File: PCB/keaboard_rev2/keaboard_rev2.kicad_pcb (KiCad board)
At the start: 2 copper layers, 141.9 x 93.7 mm, 61 parts, among them K01 KEYSW, K02 KEYSW, K03 KEYSW, K04 KEYSW, K05 KEYSW, K06 KEYSW, K07 KEYSW, K08 KEYSW, K09 KEYSW, K10 KEYSW, K11 KEYSW, K12 KEYSW, K13 KEYSW, K14 KEYSW, K15 KEYSW, K16 KEYSW, K17 KEYSW, K18 KEYSW, K19 KEYSW, K20 KEYSW, K21 KEYSW, K22 KEYSW, K23 KEYSW, K24 KEYSW, K25 KEYSW, U1 ProMicro

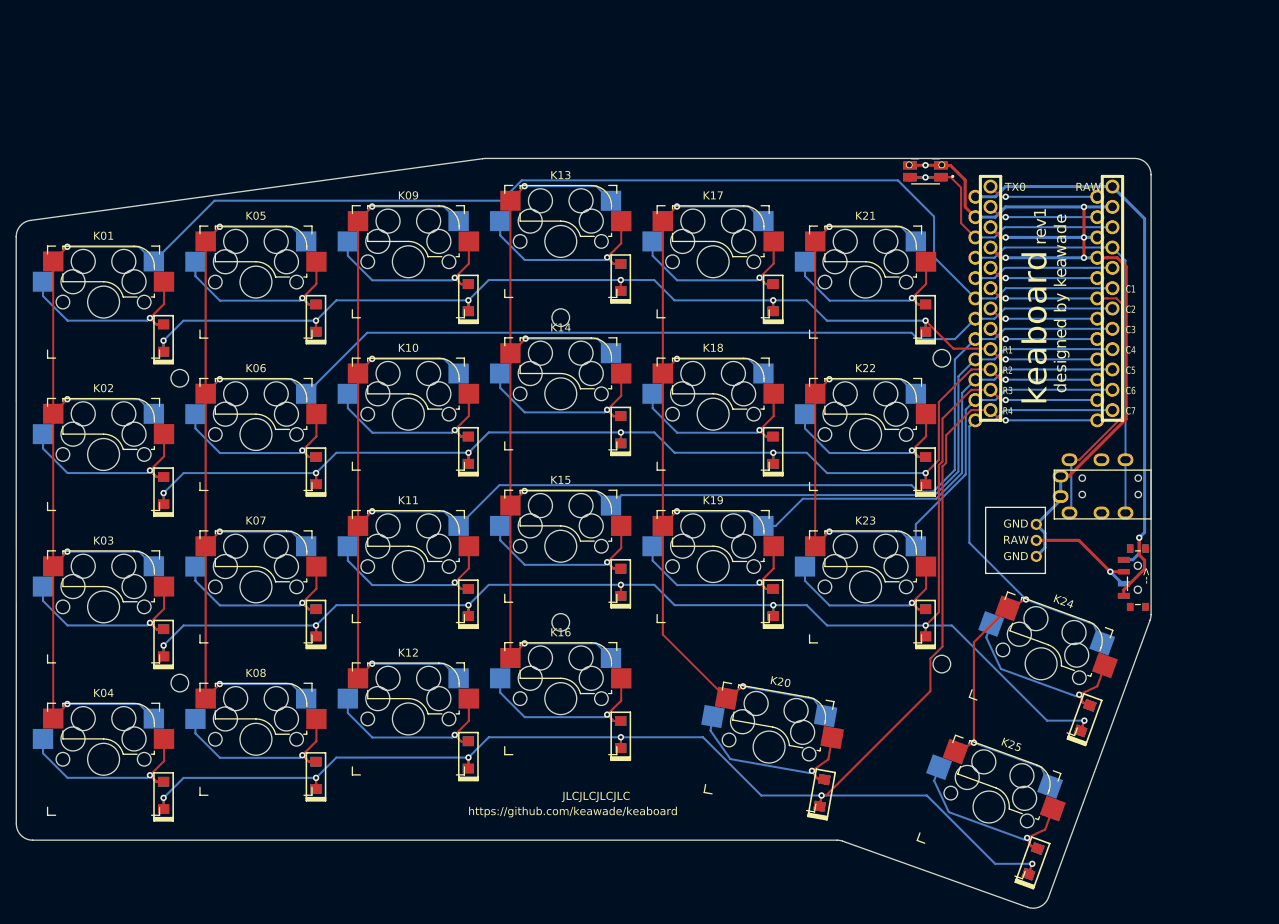
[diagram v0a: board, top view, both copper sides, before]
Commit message: WIP rev2
Just traces remaining
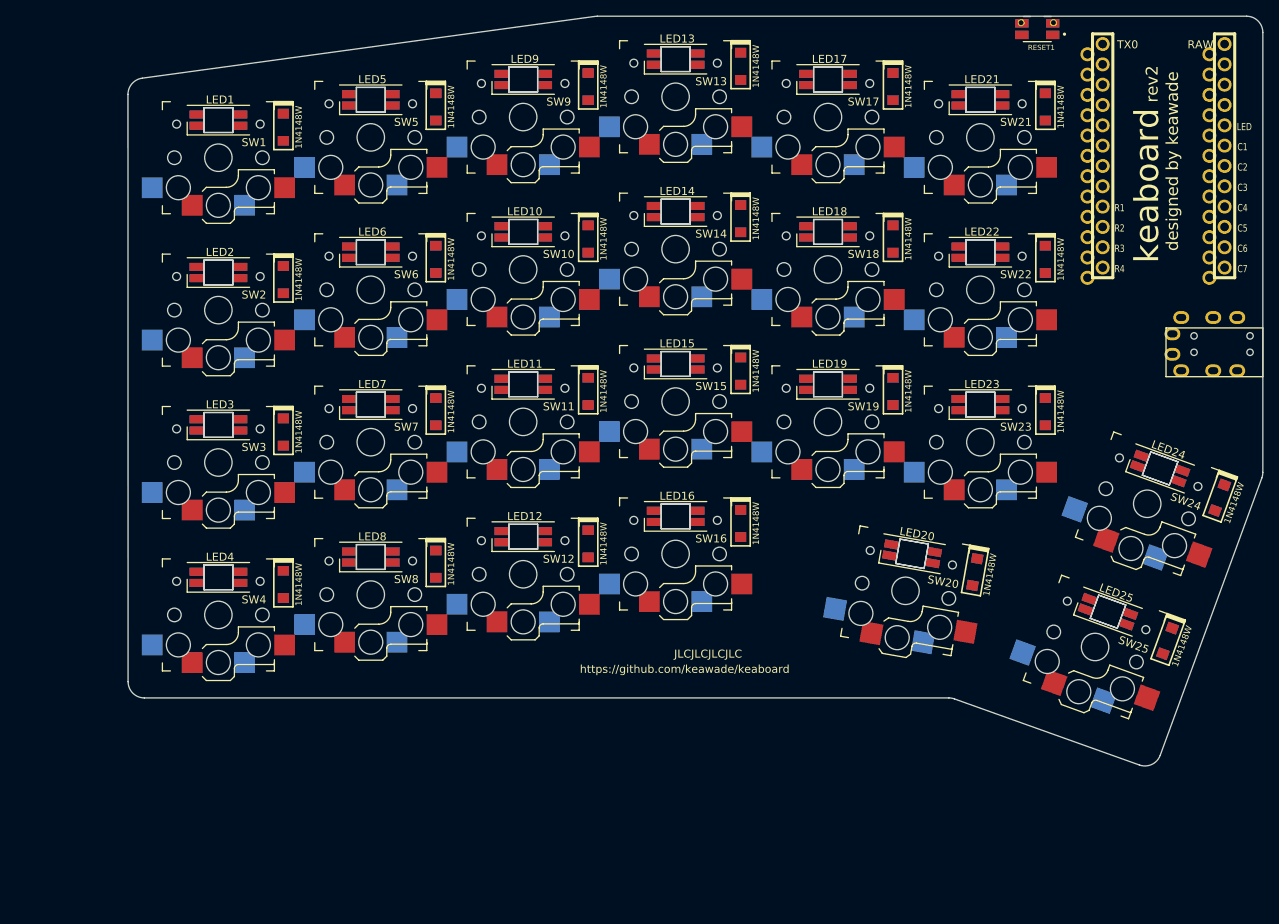
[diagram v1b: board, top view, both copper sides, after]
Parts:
- removed BAT1: Battery, parts:DF3A-3P-2DS_reversible
- removed D01, D02, D03, D04, D05, D06, D07, D08, D09: D, parts:D_SOD123_reversible
- removed K01, K02, K03, K04, K05, K06, K07, K08, K09, K10, K11, K12, K13, K14, K15, K16, K17, K18, K19, K20, K21, K22, K23, K24, K25: KEYSW, parts:Kailh_socket_MX_reversible
- removed REF** (x6): MountingHole_2.2mm_M2, MountingHole:MountingHole_2.2mm_M2
- removed SW_PWR1: SW_Push_SPDT, parts:SW_PCM12SMTR_reversible
- removed SW_RST1: SW_EVQ-9P701P, parts:SW_EVQ-9P701P_reversible
- removed TRRS1: TRRS Jack, parts:TRRS-PJ-320A_reversible
- added D1: 1N4148W, parts:D_SOD123_reversible, F.Cu at (63.2, 53.3)
- added D2: 1N4148W, parts:D_SOD123_reversible, F.Cu at (63.2, 72.3)
- added D3: 1N4148W, parts:D_SOD123_reversible, F.Cu at (63.2, 91.4)
- added D4: 1N4148W, parts:D_SOD123_reversible, F.Cu at (63.2, 110.4)
- added D5: 1N4148W, parts:D_SOD123_reversible, F.Cu at (82.3, 50.7)
- added D6: 1N4148W, parts:D_SOD123_reversible, F.Cu at (82.3, 69.8)
- added D7: 1N4148W, parts:D_SOD123_reversible, F.Cu at (82.3, 88.8)
- added D8: 1N4148W, parts:D_SOD123_reversible, F.Cu at (82.3, 107.9)
- added D9: 1N4148W, parts:D_SOD123_reversible, F.Cu at (101.3, 48.2)
- added J1: AudioJack4, parts:TRRS-PJ-320A_reversible, F.Cu at (185.7, 81.2)
- added LED1: SK6812MINI, parts:YS-SK6812MINI-E_reversible, F.Cu at (55.1, 52.4)
- added LED10: SK6812MINI, parts:YS-SK6812MINI-E_reversible, F.Cu at (93.2, 66.4)
- added LED11: SK6812MINI, parts:YS-SK6812MINI-E_reversible, F.Cu at (93.2, 85.4)
- added LED12: SK6812MINI, parts:YS-SK6812MINI-E_reversible, F.Cu at (93.2, 104.5)
- added LED13: SK6812MINI, parts:YS-SK6812MINI-E_reversible, F.Cu at (112.3, 44.8)
- added LED14: SK6812MINI, parts:YS-SK6812MINI-E_reversible, F.Cu at (112.3, 63.8)
- added LED15: SK6812MINI, parts:YS-SK6812MINI-E_reversible, F.Cu at (112.3, 82.9)
- added LED16: SK6812MINI, parts:YS-SK6812MINI-E_reversible, F.Cu at (112.3, 101.9)
- added LED17: SK6812MINI, parts:YS-SK6812MINI-E_reversible, F.Cu at (131.3, 47.3)
- added LED18: SK6812MINI, parts:YS-SK6812MINI-E_reversible, F.Cu at (131.3, 66.4)
- added LED19: SK6812MINI, parts:YS-SK6812MINI-E_reversible, F.Cu at (131.3, 85.4)
- added LED2: SK6812MINI, parts:YS-SK6812MINI-E_reversible, F.Cu at (55.1, 71.5)
- added LED20: SK6812MINI, parts:YS-SK6812MINI-E_reversible, F.Cu at (141.8, 106.6)
- added LED21: SK6812MINI, parts:YS-SK6812MINI-E_reversible, F.Cu at (150.4, 49.9)
- added LED22: SK6812MINI, parts:YS-SK6812MINI-E_reversible, F.Cu at (150.4, 68.9)
- added LED23: SK6812MINI, parts:YS-SK6812MINI-E_reversible, F.Cu at (150.4, 88.0)
- added LED24: SK6812MINI, parts:YS-SK6812MINI-E_reversible, F.Cu at (172.8, 95.9)
- added LED25: SK6812MINI, parts:YS-SK6812MINI-E_reversible, F.Cu at (166.3, 113.8)
- added LED3: SK6812MINI, parts:YS-SK6812MINI-E_reversible, F.Cu at (55.1, 90.5)
- added LED4: SK6812MINI, parts:YS-SK6812MINI-E_reversible, F.Cu at (55.1, 109.6)
- added LED5: SK6812MINI, parts:YS-SK6812MINI-E_reversible, F.Cu at (74.2, 49.9)
- added LED6: SK6812MINI, parts:YS-SK6812MINI-E_reversible, F.Cu at (74.2, 68.9)
- added LED7: SK6812MINI, parts:YS-SK6812MINI-E_reversible, F.Cu at (74.2, 88.0)
- added LED8: SK6812MINI, parts:YS-SK6812MINI-E_reversible, F.Cu at (74.2, 107.0)
- added LED9: SK6812MINI, parts:YS-SK6812MINI-E_reversible, F.Cu at (93.2, 47.3)
- added RESET1: SW_Push, parts:SW_EVQ-9P701P_reversible, F.Cu at (157.5, 41.0)
- added SW1: SW_Push, keyswitches:Kailh_socket_PG1350_reversible, F.Cu at (55.1, 57.1)
- added SW10: SW_Push, keyswitches:Kailh_socket_PG1350_reversible, F.Cu at (93.2, 71.1)
- added SW11: SW_Push, keyswitches:Kailh_socket_PG1350_reversible, F.Cu at (93.2, 90.1)
- added SW12: SW_Push, keyswitches:Kailh_socket_PG1350_reversible, F.Cu at (93.2, 109.2)
- added SW13: SW_Push, keyswitches:Kailh_socket_PG1350_reversible, F.Cu at (112.3, 49.5)
- added SW14: SW_Push, keyswitches:Kailh_socket_PG1350_reversible, F.Cu at (112.3, 68.5)
- added SW15: SW_Push, keyswitches:Kailh_socket_PG1350_reversible, F.Cu at (112.3, 87.6)
- added SW16: SW_Push, keyswitches:Kailh_socket_PG1350_reversible, F.Cu at (112.3, 106.6)
- added SW17: SW_Push, keyswitches:Kailh_socket_PG1350_reversible, F.Cu at (131.3, 52.0)
- added SW18: SW_Push, keyswitches:Kailh_socket_PG1350_reversible, F.Cu at (131.3, 71.1)
- added SW19: SW_Push, keyswitches:Kailh_socket_PG1350_reversible, F.Cu at (131.3, 90.1)
- added SW2: SW_Push, keyswitches:Kailh_socket_PG1350_reversible, F.Cu at (55.1, 76.1)
- added SW20: SW_Push, keyswitches:Kailh_socket_PG1350_reversible, F.Cu at (141.0, 111.2)
- added SW21: SW_Push, keyswitches:Kailh_socket_PG1350_reversible, F.Cu at (150.4, 54.6)
- added SW22: SW_Push, keyswitches:Kailh_socket_PG1350_reversible, F.Cu at (150.4, 73.6)
- added SW23: SW_Push, keyswitches:Kailh_socket_PG1350_reversible, F.Cu at (150.4, 92.7)
- added SW24: SW_Push, keyswitches:Kailh_socket_PG1350_reversible, F.Cu at (171.2, 100.4)
- added SW25: SW_Push, keyswitches:Kailh_socket_PG1350_reversible, F.Cu at (164.7, 118.3)
- added SW3: SW_Push, keyswitches:Kailh_socket_PG1350_reversible, F.Cu at (55.1, 95.2)
- added SW4: SW_Push, keyswitches:Kailh_socket_PG1350_reversible, F.Cu at (55.1, 114.2)
- added SW5: SW_Push, keyswitches:Kailh_socket_PG1350_reversible, F.Cu at (74.2, 54.6)
- added SW6: SW_Push, keyswitches:Kailh_socket_PG1350_reversible, F.Cu at (74.2, 73.6)
- added SW7: SW_Push, keyswitches:Kailh_socket_PG1350_reversible, F.Cu at (74.2, 92.7)
- added SW8: SW_Push, keyswitches:Kailh_socket_PG1350_reversible, F.Cu at (74.2, 111.7)
- added SW9: SW_Push, keyswitches:Kailh_socket_PG1350_reversible, F.Cu at (93.2, 52.0)
- D10, D11, D12, D13, D14, D15, D16, D17, D18, D19, D20, D21, D22, D23, D24, D25: value D -> 1N4148W
- moved D20 33.6 mm to (149.7, 108.9), turned to 80 degrees
- moved D25 32.3 mm to (173.8, 117.5), turned to 70 degrees
- moved D24 32.3 mm to (180.3, 99.6), turned to 70 degrees
- moved D21 30.3 mm to (158.5, 50.7), turned to 90 degrees
- moved D22 30.3 mm to (158.5, 69.8), turned to 90 degrees
- moved D23 30.3 mm to (158.5, 88.8), turned to 90 degrees
- moved D14 30.3 mm to (120.4, 64.7), turned to 90 degrees
- moved D15 30.3 mm to (120.4, 83.8), turned to 90 degrees
- moved D16 30.3 mm to (120.4, 102.8), turned to 90 degrees
- moved D13 30.3 mm to (120.4, 45.7), turned to 90 degrees
- moved D17 30.3 mm to (139.4, 48.2), turned to 90 degrees
- moved D10 30.3 mm to (101.3, 67.3), turned to 90 degrees
- moved D11 30.3 mm to (101.3, 86.3), turned to 90 degrees
- moved D12 30.3 mm to (101.3, 105.4), turned to 90 degrees
- moved D18 30.3 mm to (139.4, 67.3), turned to 90 degrees
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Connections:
- D10 pad 1: ROW2 -> Row2
- D11 pad 1: ROW3 -> Row3
- D12 pad 1: ROW4 -> Row4
- D13 pad 1: ROW1 -> Row1
- D14 pad 1: ROW2 -> Row2
- D15 pad 1: ROW3 -> Row3
- D16 pad 1: ROW4 -> Row4
- D17 pad 1: ROW1 -> Row1
- D18 pad 1: ROW2 -> Row2
- D19 pad 1: ROW3 -> Row3
- D20 pad 1: ROW4 -> Row4
- D21 pad 1: ROW1 -> Row1
- D22 pad 1: ROW2 -> Row2
- D23 pad 1: ROW3 -> Row3
- D24 pad 1: ROW3 -> Row3
- D25 pad 1: ROW4 -> Row4
- U1 pad 10: ROW2 -> Row3
- U1 pad 11: ROW3 -> Row4
- U1 pad 12: ROW4 -> Col1
- U1 pad 13: COL7 -> Col2
- U1 pad 14: COL6 -> Col3
- U1 pad 15: COL5 -> Col4
- U1 pad 16: COL4 -> Col5
- U1 pad 17: COL3 -> Col6
- U1 pad 18: COL2 -> Col7
- U1 pad 19: COL1 -> TRRS_T
- U1 pad 20: Net-(U1-Pad20) -> LED
- U1 pad 21: VCC -> Net-(U1-Pad21)
- U1 pad 5: Net-(U1-Pad5) -> TRRS_R2
- U1 pad 6: SOFT_SERIAL_PIN -> Net-(U1-Pad6)
- U1 pad 8: Net-(U1-Pad8) -> Row1
- U1 pad 9: ROW1 -> Row2
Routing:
- net COL1: track 247.3 -> 0.00 mm, vias 4 -> 0
- net COL2: track 219.5 -> 0.00 mm, vias 4 -> 0
- net COL3: track 214.3 -> 0.00 mm, vias 4 -> 0
- net ROW4: track 207.2 -> 0.00 mm, vias 7 -> 0
- net ROW3: track 192.5 -> 0.00 mm, vias 8 -> 0
- net COL4: track 191.4 -> 0.00 mm, vias 4 -> 0
- net COL5: track 177.0 -> 0.00 mm, vias 4 -> 0
- net ROW2: track 148.5 -> 0.00 mm, vias 7 -> 0
- net ROW1: track 140.4 -> 0.00 mm, vias 7 -> 0
- net COL6: track 119.5 -> 0.00 mm, vias 3 -> 0
- net GND: track 111.3 -> 0.00 mm, vias 6 -> 0
- net COL7: track 90.1 -> 0.00 mm, vias 2 -> 0
- net RAW: track 76.3 -> 0.00 mm, vias 1 -> 0
- net VCC: track 51.5 -> 0.00 mm
- net SOFT_SERIAL_PIN: track 47.0 -> 0.00 mm, vias 1 -> 0
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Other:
- net class Default: trace_width 0.254 -> 0.25
- net class Power removed
- rule pad_to_mask_clearance: 0.05 -> 0
- board text added: "LED"
- board text added: "rev2"
- board text removed: "rev1"
